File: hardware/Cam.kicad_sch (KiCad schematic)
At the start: 1 part

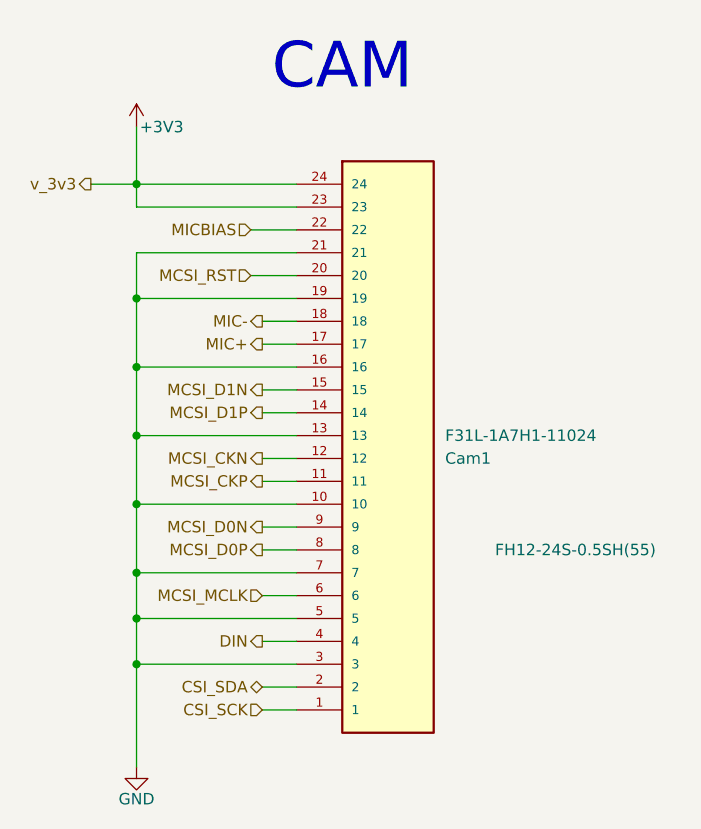
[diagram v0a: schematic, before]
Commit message: feat(Hw):Update_Schematic_And_BOM
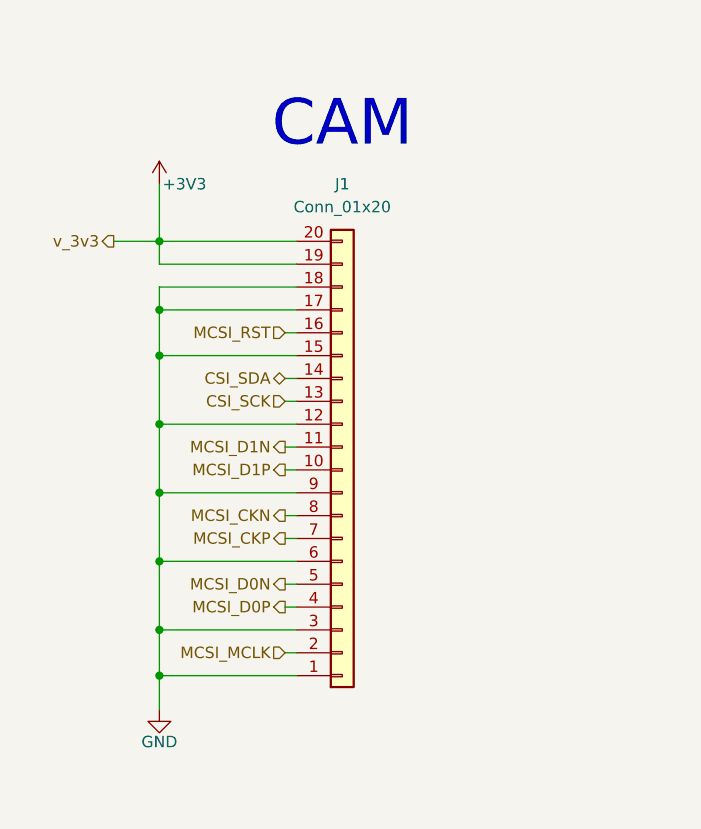
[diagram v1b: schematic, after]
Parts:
- removed Cam1: F31L-1A7H1-11024, Connector_FFC-FPC:Hirose_FH12-24S-0.5SH_1x24-1MP_P0.50mm_Horizontal, symbol F31L-1A7H1-11024:F31L-1A7H1-11024
- added J1: Conn_01x20, Connector_FFC-FPC:Hirose_FH12-20S-0.5SH_1x20-1MP_P0.50mm_Horizontal, symbol Connector_Generic:Conn_01x20
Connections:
- net +3V3: now also J1.19 (Pin_19), J1.20 (Pin_20)
- net CSI_SCK: now also J1.13 (Pin_13)
- net CSI_SDA: now also J1.14 (Pin_14)
- net GND: now also J1.1 (Pin_1), J1.12 (Pin_12), J1.15 (Pin_15), J1.17 (Pin_17), J1.18 (Pin_18), J1.3 (Pin_3), J1.6 (Pin_6), J1.9 (Pin_9)
- net MCSI_CKN: now also J1.8 (Pin_8)
- net MCSI_CKP: now also J1.7 (Pin_7)
- net MCSI_D0N: now also J1.5 (Pin_5)
- net MCSI_D0P: now also J1.4 (Pin_4)
- net MCSI_D1N: now also J1.11 (Pin_11)
- net MCSI_D1P: now also J1.10 (Pin_10)
- net MCSI_MCLK: now also J1.2 (Pin_2)
- net MCSI_RST: now also J1.16 (Pin_16)
